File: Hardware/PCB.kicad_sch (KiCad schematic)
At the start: 0 parts

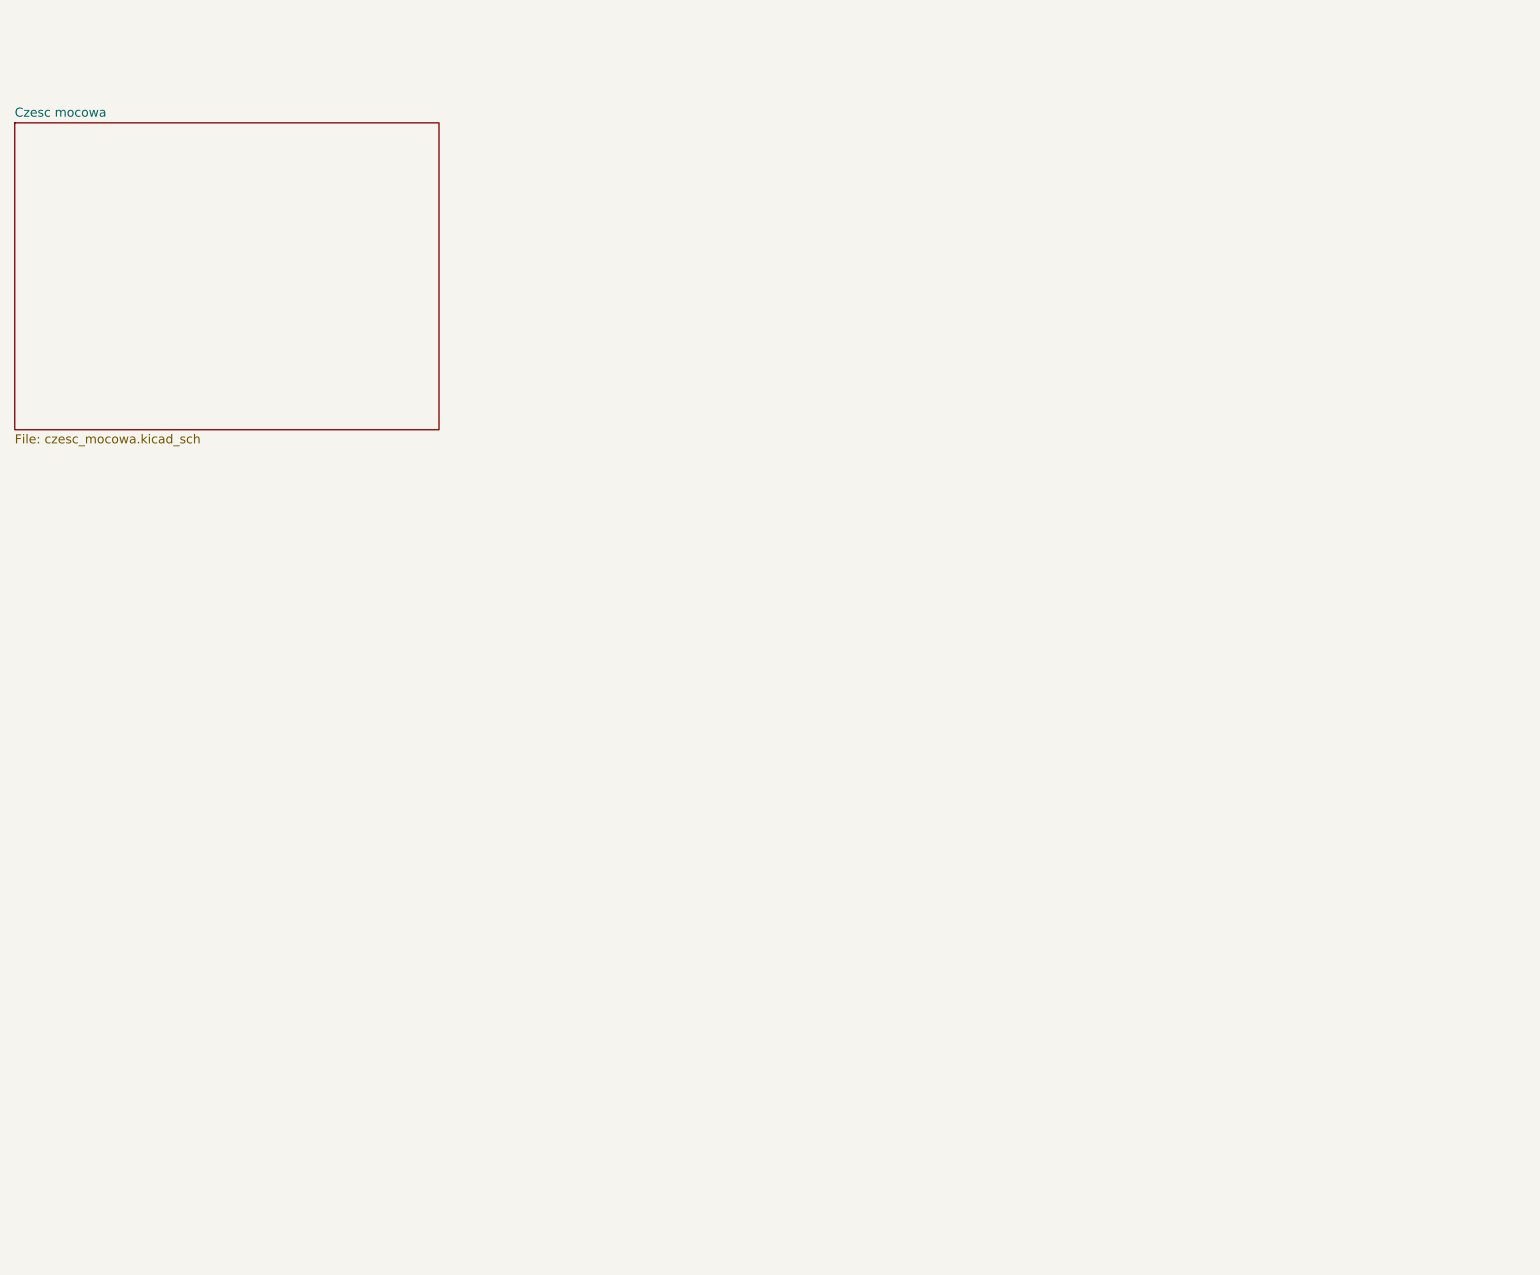
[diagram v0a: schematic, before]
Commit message: Added PCB
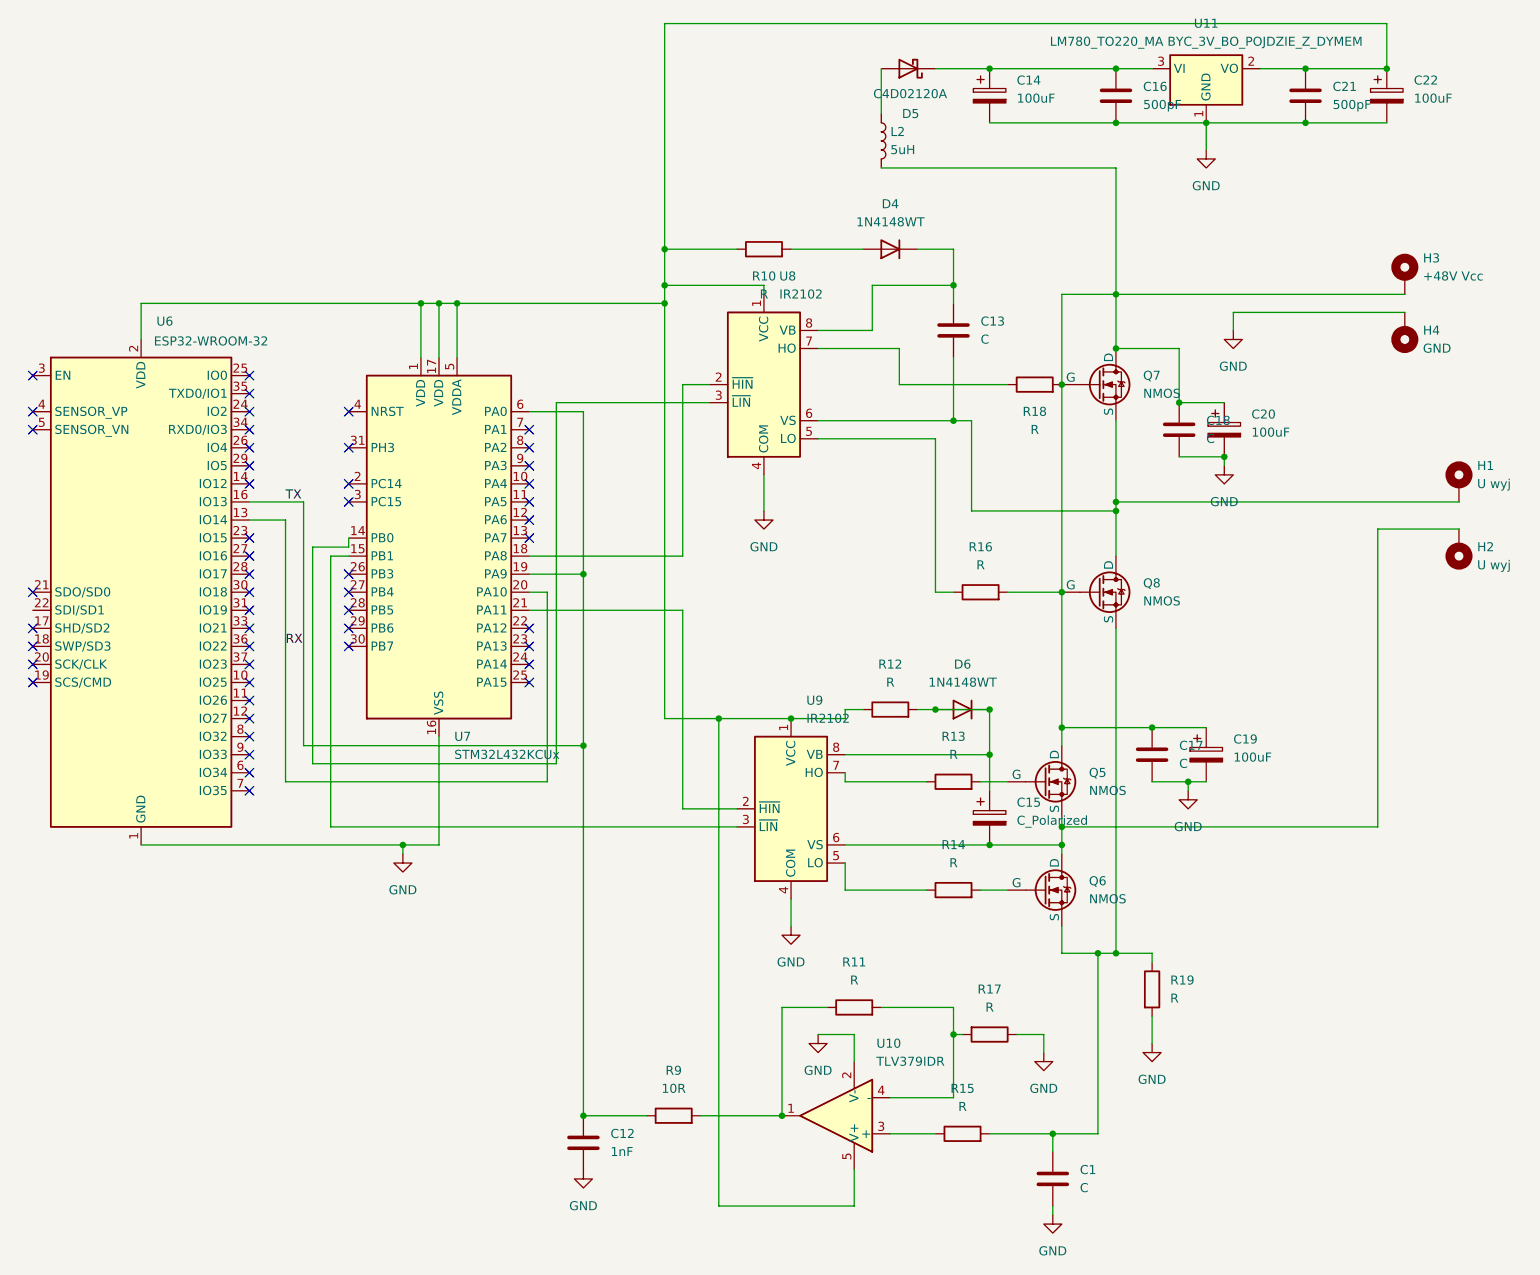
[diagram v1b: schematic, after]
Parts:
- added C1, C13, C17, C18: C, Capacitor_SMD:C_1206_3216Metric, symbol Device:C
- added C12: 1nF, Capacitor_SMD:C_1206_3216Metric, symbol Device:C
- added C14, C19, C20, C22: 100uF, Capacitor_SMD:CP_Elec_10x10, symbol Device:C_Polarized
- added C15: C_Polarized, Capacitor_SMD:CP_Elec_5x5.3, symbol Device:C_Polarized
- added C16, C21: 500pF, Capacitor_SMD:C_1206_3216Metric, symbol Device:C
- added D4, D6: 1N4148WT, Diode_SMD:D_SOD-523, symbol Diode:1N4148WT
- added D5: C4D02120A, Package_TO_SOT_THT:TO-220-2_Vertical, symbol Diode:C4D02120A
- added H1, H2: U wyj, MountingHole:MountingHole_3.2mm_M3_DIN965_Pad, symbol Mechanical:MountingHole_Pad
- added H3: +48V Vcc, MountingHole:MountingHole_3.2mm_M3_DIN965_Pad, symbol Mechanical:MountingHole_Pad
- added H4: GND, MountingHole:MountingHole_3.2mm_M3_DIN965_Pad, symbol Mechanical:MountingHole_Pad
- added L2: 5uH, Inductor_SMD:L_6.3x6.3_H3, symbol Device:L
- added Q5, Q6, Q7, Q8: NMOS, Package_TO_SOT_THT:TO-220-3_Horizontal_TabUp, symbol Simulation_SPICE:NMOS
- added R10, R11, R12, R13, R14, R15, R16, R17, R18, R19: R, Resistor_SMD:R_1210_3225Metric, symbol Device:R
- added R9: 10R, Resistor_SMD:R_1210_3225Metric, symbol Device:R
- added U10: TLV379IDR, Package_TO_SOT_SMD:SOT-23-5, symbol Amplifier_Operational:TLV2371DBV
- added U11: LM780_TO220_MA BYC_3V_BO_POJDZIE_Z_DYMEM, Package_TO_SOT_THT:TO-220-3_Horizontal_TabUp, symbol Regulator_Linear:LD1117S33TR_SOT223
- added U6: ESP32-WROOM-32, RF_Module:ESP32-WROOM-32, symbol RF_Module:ESP32-WROOM-32
- added U7: STM32L432KCUx, Package_DFN_QFN:QFN-32-1EP_5x5mm_P0.5mm_EP3.45x3.45mm, symbol MCU_ST_STM32L4:STM32L432KCUx
- added U8, U9: IR2102, Package_SO:SOIC-8-1EP_3.9x4.9mm_P1.27mm_EP2.29x3mm, symbol Driver_FET:IR2102
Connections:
- new net: C15.1, D6.1 (K), D6.2 (A), R12.2, U9.8 (VB)
- new net: C15.2, H2.1, Q5.3 (S), Q6.1 (D), U9.6 (VS)
- new net: C13.1, D4.1 (K), U8.8 (VB)
- new net: D4.2 (A), R10.2
- new net: R13.1, U9.7 (HO)
- new net: Q5.2 (G), R13.2
- new net: R16.1, U8.5 (LO)
- new net: C17.1, C18.1, C19.1, C20.1, H3.1, L2.2, Q5.1 (D), Q7.1 (D), Q7.2 (G), Q8.2 (G), R16.2, R18.2
- new net: C21.1, C22.1, R10.1, R12.1, U10.5 (V+), U11.2 (VO), U6.2 (VDD), U7.1 (VDD), U7.17 (VDD), U7.5 (VDDA), U8.1 (VCC), U9.1 (VCC)
- new net: C13.2, H1.1, Q7.3 (S), Q8.1 (D), U8.6 (VS)
- new net: R11.2, R17.2, U10.4 (-)
- new net: Q6.2 (G), R14.2
- new net: C1.1, Q6.3 (S), Q8.3 (S), R15.2, R19.1
- new net: R14.1, U9.5 (LO)
- new net: R11.1, R9.2, U10.1
- new net: C14.1, C16.1, D5.1 (K), U11.3 (VI)
- new net: D5.2 (A), L2.1
- new net: R18.1, U8.7 (HO)
- new net: U7.14 (PB0), U8.3 (~{LIN})
- new net: U7.15 (PB1), U9.3 (~{LIN})
- new net: U7.18 (PA8), U8.2 (~{HIN})
- new net: U7.21 (PA11), U9.2 (~{HIN})
- new net: R15.1, U10.3 (+)
- new net GND: C1.2, C12.2, C14.2, C16.2, C17.2, C18.2, C19.2, C20.2, C21.2, C22.2, H4.1, R17.1, R19.2, U10.2 (V-), U11.1 (GND), U6.1 (GND), U6.15 (GND), U6.38 (GND), U6.39 (GND), U7.16 (VSS), U7.32 (VSS), U7.33 (VSS), U8.4 (COM), U9.4 (COM)
- new net RX: U6.13 (IO14), U7.20 (PA10)
- new net TX: C12.1, R9.1, U6.16 (IO13), U7.19 (PA9), U7.6 (PA0)
- no-connect marks 0 -> 50
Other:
- removed sheet Czesc mocowa
